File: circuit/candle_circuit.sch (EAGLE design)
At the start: 25 parts, among them IC1 TINY10P, SW1 KMR2, SW2 KMR2, X1 ESP-12

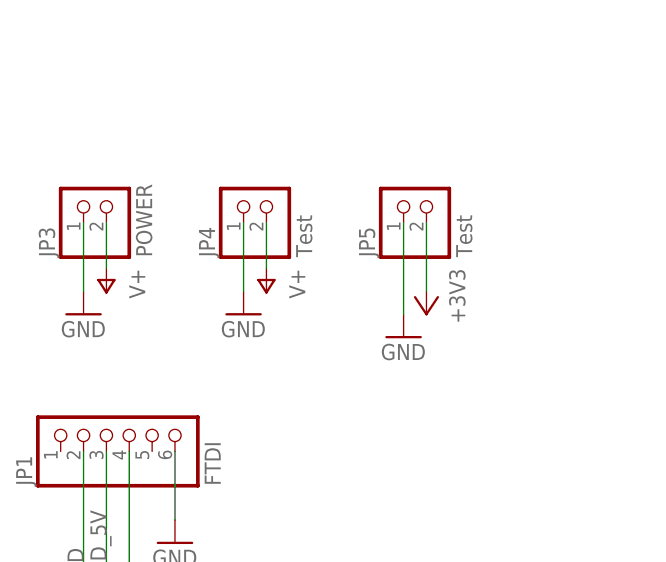
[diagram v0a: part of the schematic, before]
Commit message: Board updates
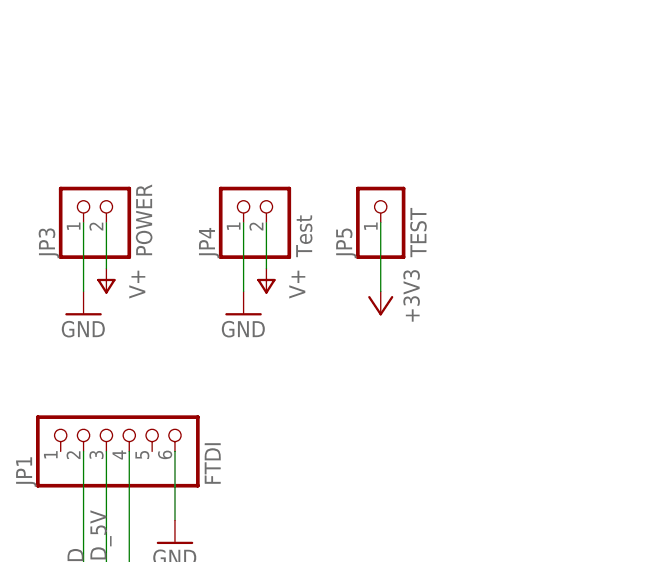
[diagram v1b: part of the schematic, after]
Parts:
- JP5: value Test -> TEST; device microbuilder:HEADER-1X2 -> pinhead:PINHD-1X1
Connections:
- net +3V3: now also JP5.1; no longer JP5.2
- net GND: no longer JP5.1
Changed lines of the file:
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@@
 <part name="R4" library="adafruit" deviceset="R-US_" device="R0603" value="10k"/>
 <part name="JP4" library="microbuilder" deviceset="HEADER-1X2" device="" value="Test"/>
-<part name="JP5" library="microbuilder" deviceset="HEADER-1X2" device="" value="Test"/>
 <part name="GND8" library="supply1" deviceset="GND" device=""/>
-<part name="GND12" library="supply1" deviceset="GND" device=""/>
 <part name="P+4" library="supply1" deviceset="V+" device=""/>
+<part name="JP5" library="pinhead" deviceset="PINHD-1X1" device="" value="TEST"/>
 <part name="+3V8" library="supply1" deviceset="+3V3" device=""/>
 </parts>
@@
 <instance part="R4" gate="G$1" x="-40.64" y="81.28" rot="R270"/>
 <instance part="JP4" gate="G$1" x="101.6" y="93.98" rot="R90"/>
-<instance part="JP5" gate="G$1" x="119.38" y="93.98" rot="R90"/>
 <instance part="GND8" gate="1" x="99.06" y="81.28"/>
-<instance part="GND12" gate="1" x="116.84" y="78.74"/>
 <instance part="P+4" gate="1" x="101.6" y="83.82" rot="R180"/>
-<instance part="+3V8" gate="G$1" x="119.38" y="81.28" rot="R180"/>
+<instance part="JP5" gate="G$1" x="114.3" y="93.98" rot="R90"/>
+<instance part="+3V8" gate="G$1" x="114.3" y="81.28" rot="R180"/>
 </instances>
 <busses>
@@
 <wire x1="99.06" y1="91.44" x2="99.06" y2="83.82" width="0.1524" layer="91"/>
 </segment>
-<segment>
-<pinref part="JP5" gate="G$1" pin="1"/>
-<pinref part="GND12" gate="1" pin="GND"/>
-<wire x1="116.84" y1="91.44" x2="116.84" y2="81.28" width="0.1524" layer="91"/>
-</segment>
 </net>
 <net name="+3V3" class="0">
@@
 </segment>
 <segment>
-<pinref part="JP5" gate="G$1" pin="2"/>
+<pinref part="JP5" gate="G$1" pin="1"/>
 <pinref part="+3V8" gate="G$1" pin="+3V3"/>
-<wire x1="119.38" y1="91.44" x2="119.38" y2="83.82" width="0.1524" layer="91"/>
+<wire x1="114.3" y1="91.44" x2="114.3" y2="83.82" width="0.1524" layer="91"/>
 </segment>
 </net>
